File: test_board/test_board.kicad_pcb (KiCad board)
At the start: 2 copper layers, 8 parts, among them IC1 TC118S, J1 MotorConnection, U1 ACS712xLCTR-05B

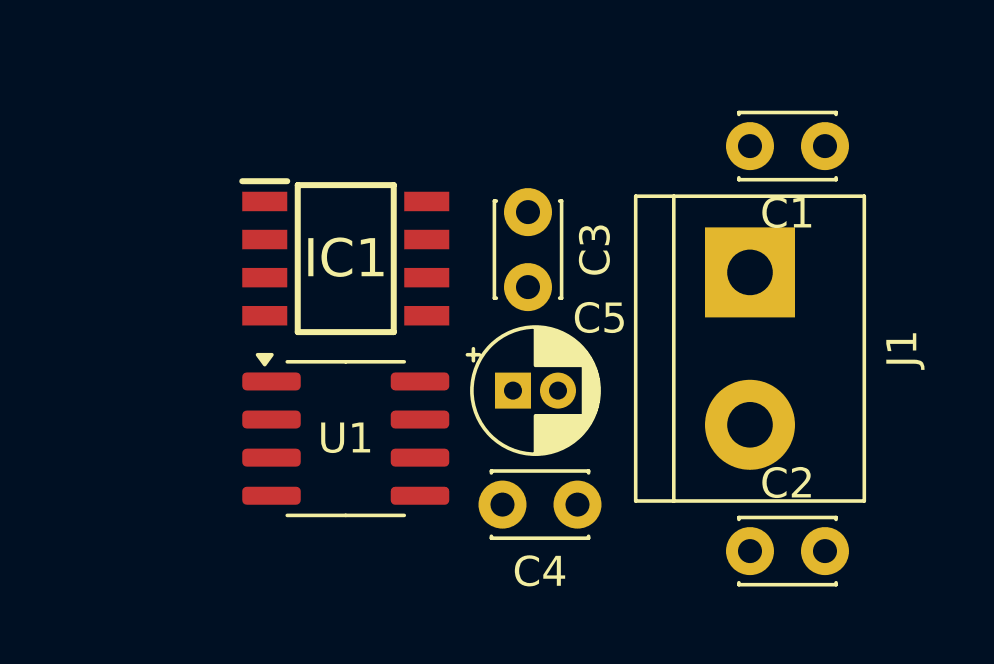
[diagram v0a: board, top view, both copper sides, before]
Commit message: Improved MG-X
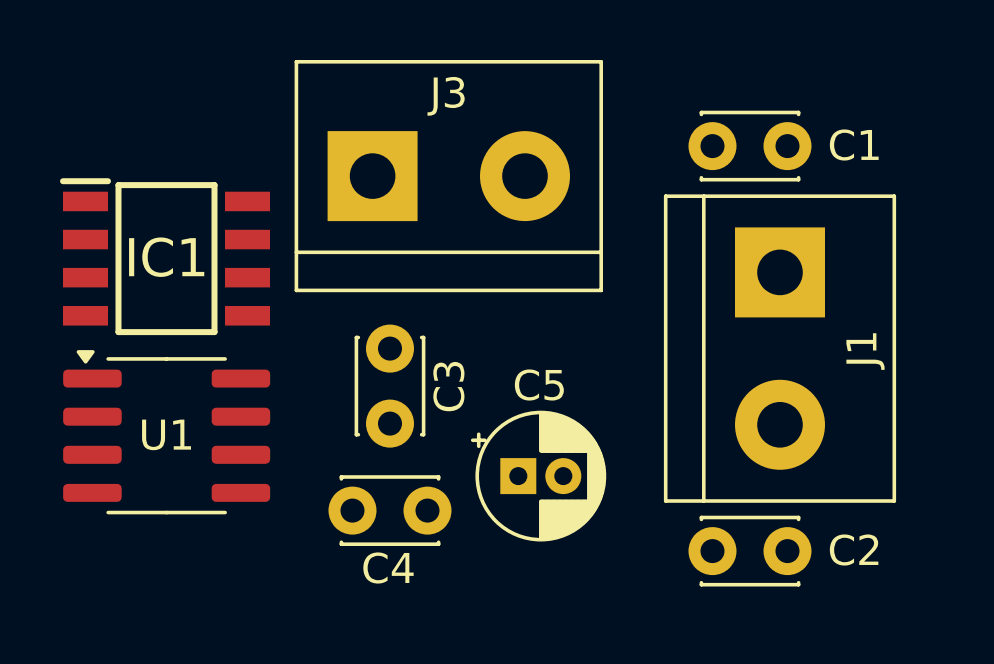
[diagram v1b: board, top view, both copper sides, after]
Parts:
- added J3: PowerSupply, TerminalBlock:TerminalBlock_bornier-2_P5.08mm, F.Cu at (132.4, 88.2)
- moved C4 7.50 mm to (131.8, 99.4), turned to 0 degrees
- moved C3 6.47 mm to (133.0, 94.0)
- moved IC1 5.98 mm to (125.5, 91.0)
- moved U1 5.97 mm to (125.6, 96.9)
- moved C5 2.86 mm to (137.3, 98.2)
- moved C1 1.25 mm to (146.2, 87.2)
- moved C2 1.25 mm to (143.8, 100.8)
- moved J1 1.00 mm to (146.0, 91.5)

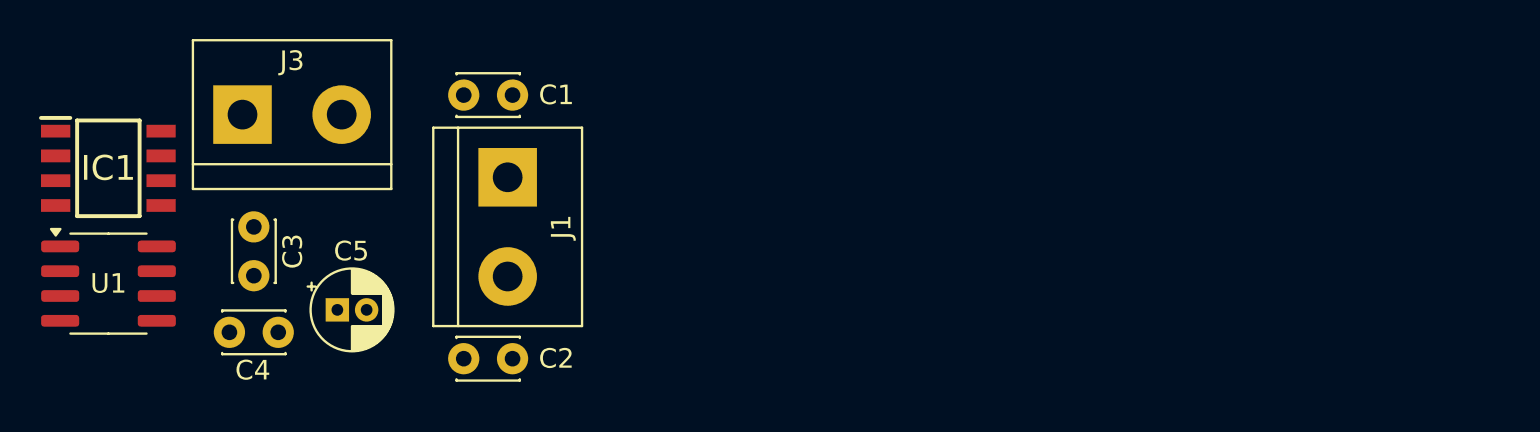
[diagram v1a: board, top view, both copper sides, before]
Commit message: Minor changes
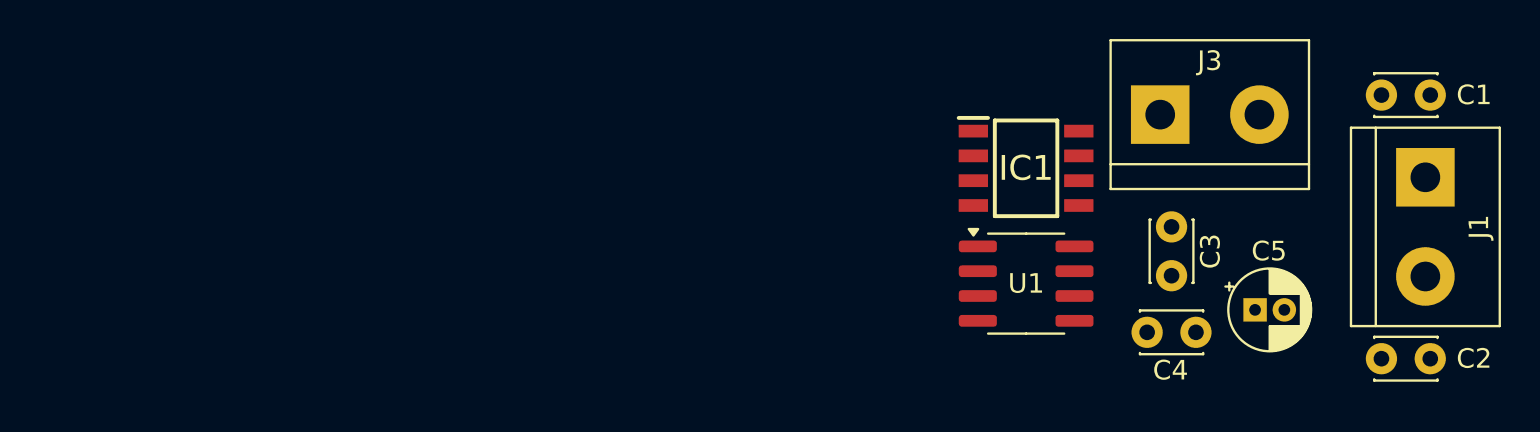
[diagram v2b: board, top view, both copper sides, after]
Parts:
- moved IC1 47.0 mm to (172.6, 91.0)
- moved C1 47.0 mm to (193.2, 87.2)
- moved C2 47.0 mm to (190.8, 100.8)
- moved C3 47.0 mm to (180.0, 94.0)
- moved C4 47.0 mm to (178.8, 99.4)
- moved C5 47.0 mm to (184.3, 98.2)
- moved J1 47.0 mm to (193.0, 91.5)
- moved J3 47.0 mm to (179.4, 88.2)
- moved U1 47.0 mm to (172.6, 96.9)
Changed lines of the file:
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@@
 	(footprint "Package_SO:SOIC-8_3.9x4.9mm_P1.27mm"
 		(layer "F.Cu")
-		(at 125.555 96.905)
+		(at 172.555 96.905)
 		(descr "SOIC, 8 Pin (JEDEC MS-012AA, https://www.analog.com/media/en/package-pcb-resources/package/pkg_pdf/soic_narrow-r/r_8.pdf), generated with kicad-footprint-generator ipc_gullwing_generator.py")
 		(tags "SOIC SO")
@@
 	(footprint "Capacitor_THT:C_Disc_D3.0mm_W2.0mm_P2.50mm"
 		(layer "F.Cu")
-		(at 133 94 -90)
+		(at 180 94 -90)
 		(descr "C, Disc series, Radial, pin pitch=2.50mm, , diameter*width=3*2mm^2, Capacitor")
 		(tags "C Disc series Radial pin pitch 2.50mm  diameter 3mm width 2mm Capacitor")
@@
 	(footprint "Capacitor_THT:C_Disc_D3.0mm_W2.0mm_P2.50mm"
 		(layer "F.Cu")
-		(at 143.75 100.75)
+		(at 190.75 100.75)
 		(descr "C, Disc series, Radial, pin pitch=2.50mm, , diameter*width=3*2mm^2, Capacitor")
 		(tags "C Disc series Radial pin pitch 2.50mm  diameter 3mm width 2mm Capacitor")
@@
 	(footprint "Capacitor_THT:C_Disc_D3.0mm_W2.0mm_P2.50mm"
 		(layer "F.Cu")
-		(at 146.25 87.25 180)
+		(at 193.25 87.25 180)
 		(descr "C, Disc series, Radial, pin pitch=2.50mm, , diameter*width=3*2mm^2, Capacitor")
 		(tags "C Disc series Radial pin pitch 2.50mm  diameter 3mm width 2mm Capacitor")
@@
 	(footprint "TerminalBlock:TerminalBlock_bornier-2_P5.08mm"
 		(layer "F.Cu")
-		(at 132.42 88.25)
+		(at 179.42 88.25)
 		(descr "simple 2-pin terminal block, pitch 5.08mm, revamped version of bornier2")
 		(tags "terminal block bornier2")
@@
 	(footprint "TerminalBlock:TerminalBlock_bornier-2_P5.08mm"
 		(layer "F.Cu")
-		(at 146 91.46 -90)
+		(at 193 91.46 -90)
 		(descr "simple 2-pin terminal block, pitch 5.08mm, revamped version of bornier2")
 		(tags "terminal block bornier2")
@@
 	(footprint "Capacitor_THT:C_Disc_D3.0mm_W2.0mm_P2.50mm"
 		(layer "F.Cu")
-		(at 131.75 99.4)
+		(at 178.75 99.4)
 		(descr "C, Disc series, Radial, pin pitch=2.50mm, , diameter*width=3*2mm^2, Capacitor")
 		(tags "C Disc series Radial pin pitch 2.50mm  diameter 3mm width 2mm Capacitor")
 		(property "Reference" "C4"
-			(at 1.2 1.95 360)
+			(at 1.2 1.95 0)
 			(layer "F.SilkS")
 			(effects
@@
 		)
 		(property "Value" "100nF"
-			(at 1.25 2.25 360)
+			(at 1.25 2.25 0)
 			(layer "F.Fab")
 			(effects
@@
 		)
 		(fp_text user "${REFERENCE}"
-			(at 1.25 0 360)
+			(at 1.25 0 0)
 			(layer "F.Fab")
 			(effects
@@
 	(footprint "Capacitor_THT:CP_Radial_D4.0mm_P1.50mm"
 		(layer "F.Cu")
-		(at 137.277401 98.25)
+		(at 184.277401 98.25)
 		(descr "CP, Radial series, Radial, pin pitch=1.50mm, , diameter=4mm, Electrolytic Capacitor")
 		(tags "CP Radial series Radial pin pitch 1.50mm  diameter 4mm Electrolytic Capacitor")
@@
 	(footprint "TC118S:SOIC127P600X155-8N"
 		(layer "F.Cu")
-		(at 125.55 91)
+		(at 172.55 91)
 		(descr "sop8")
 		(tags "Integrated Circuit")
@@
 	)
 	(gr_rect
-		(start 120.5 84)
-		(end 150.5 104)
+		(start 98 69)
+		(end 198 119)
 		(stroke
 			(width 0.05)
